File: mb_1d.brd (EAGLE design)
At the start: 100 x 80 mm, 59 parts, among them CON1 1013279X_AMPHENOL_2X25, CON2 1013279X_AMPHENOL_2X25, U1 TPS61040, U10 TPS610981, U2 MAX5394, U3 TPS61040, U4 74HC4050, U5 RFD77101, U6 MAX5394, U7 MAX5026EUT+T, U8 MAX5394, U9 HEADER_5X2_SMD_1.27MM

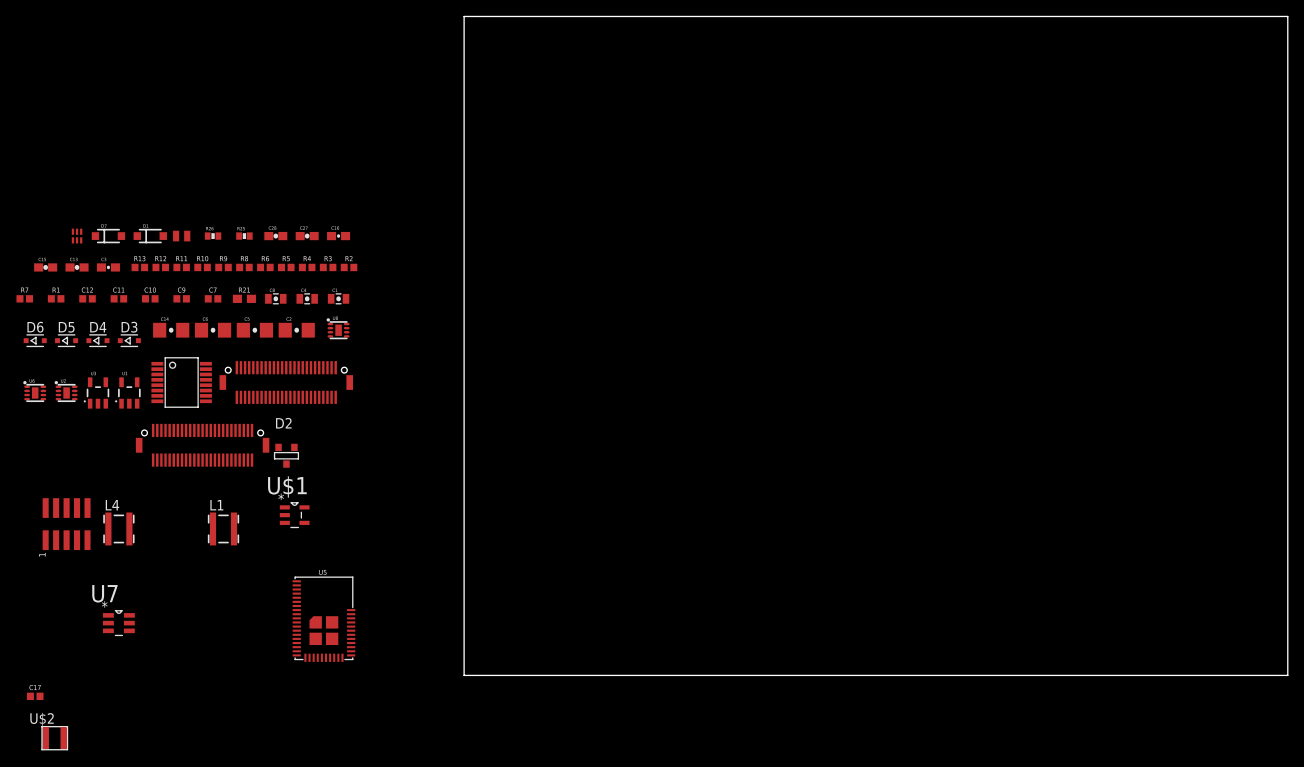
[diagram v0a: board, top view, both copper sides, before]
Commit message: Routed Simblee
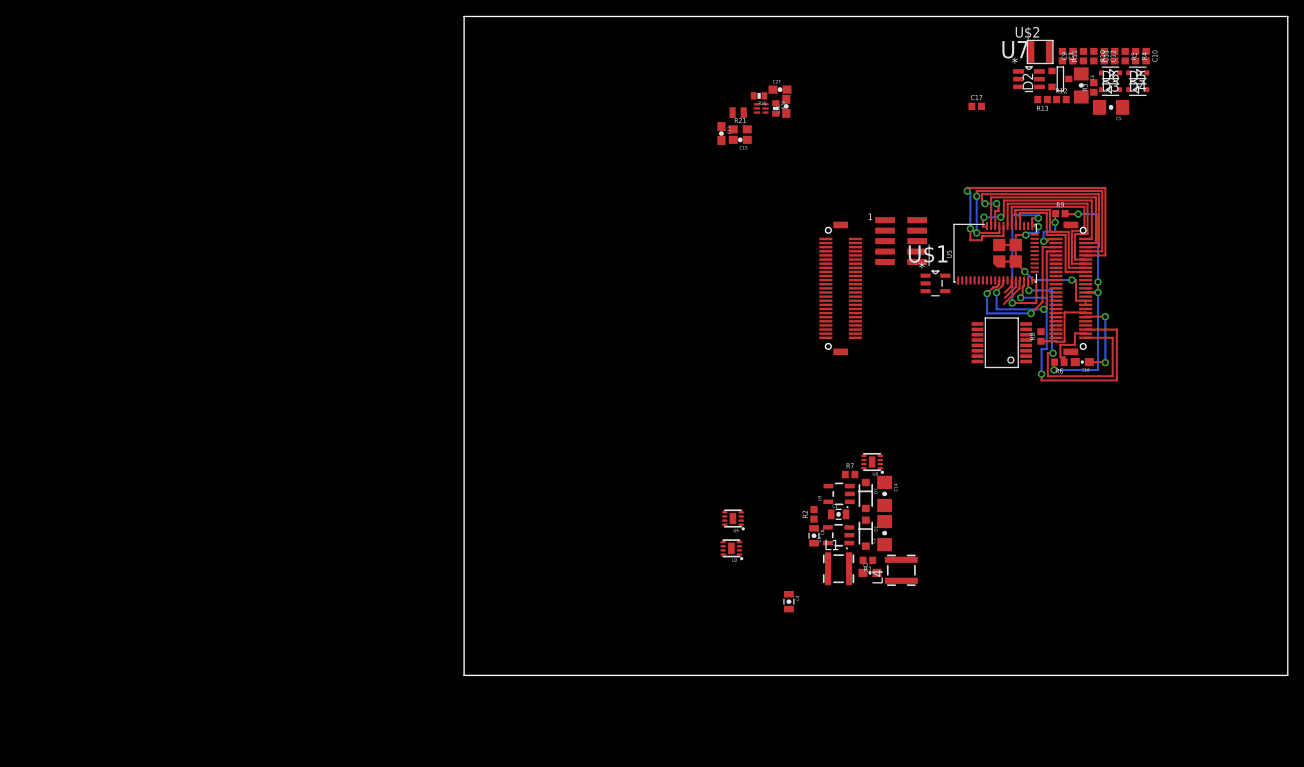
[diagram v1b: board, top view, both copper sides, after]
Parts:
- moved U$2 145.8 mm to (68.8, 75.7)
- moved C17 134.9 mm to (62.2, 69.1)
- moved D6 134.1 mm to (78.5, 71.1)
- moved D5 133.6 mm to (81.8, 71.1)
- moved D4 130.4 mm to (81.8, 73.2), turned to 180 degrees
- moved U7 128.7 mm to (68.6, 72.4)
- moved C12 126.9 mm to (77.7, 75.2), turned to 270 degrees
- moved C10 124.4 mm to (82.8, 75.2), turned to 270 degrees
- moved C11 124.4 mm to (79.0, 75.2), turned to 90 degrees
- moved D3 123.5 mm to (78.5, 73.2), turned to 180 degrees
- moved R11 112.4 mm to (75.2, 75.2), turned to 90 degrees
- moved C9 112.1 mm to (73.9, 75.2), turned to 90 degrees
- moved R13 111.5 mm to (70.2, 69.9), turned to 180 degrees
- moved U9 111.4 mm to (55.0, 55.3), turned to 270 degrees
- moved R12 111.2 mm to (72.5, 69.9)
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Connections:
- net CLK_CP: now also U5.17; no longer U5.32
- net RSTB_M: now also U5.18; no longer U5.31
- net SS_POT1: now also U5.14; no longer U5.26
- net SS_POT2: now also U5.15; no longer U5.27
- net SS_POT3: now also U5.16; no longer U5.28
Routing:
- net GND: track 0.00 -> 46.5 mm, vias 0 -> 6
- net SDI_LS: track 0.00 -> 39.8 mm, vias 0 -> 2
- net CLK_CP: track 0.00 -> 35.5 mm, vias 0 -> 2
- net SCK_LS: track 0.00 -> 33.2 mm, vias 0 -> 2
- net VDD: track 0.00 -> 32.3 mm, vias 0 -> 4
- net RSTB_M: track 0.00 -> 31.1 mm, vias 0 -> 2
- net MISO: track 0.00 -> 28.6 mm, vias 0 -> 2
- net TMODE_M: track 0.00 -> 23.0 mm
- net REF_CLK: track 0.00 -> 22.4 mm, vias 0 -> 2
- net HF_M: track 0.00 -> 22.0 mm
- net DLL_START_M: track 0.00 -> 21.3 mm
- net OUT16_BUF: track 0.00 -> 20.4 mm, vias 0 -> 2
- net REF_CLK_BUF: track 0.00 -> 18.1 mm, vias 0 -> 2
- net DLL_SAMP_M: track 0.00 -> 17.6 mm
- net DLL_EN_M: track 0.00 -> 16.8 mm
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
